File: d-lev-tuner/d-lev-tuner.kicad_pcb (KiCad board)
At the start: 4 copper layers, 88.7 x 68.4 mm, 40 parts, among them J1 S6B-PH-SM4-TB, U1 STP08CP05, U2 STP08CP05, U3 AP2112K-3.3, U4 STP08CP05, U5 DSM7TA56

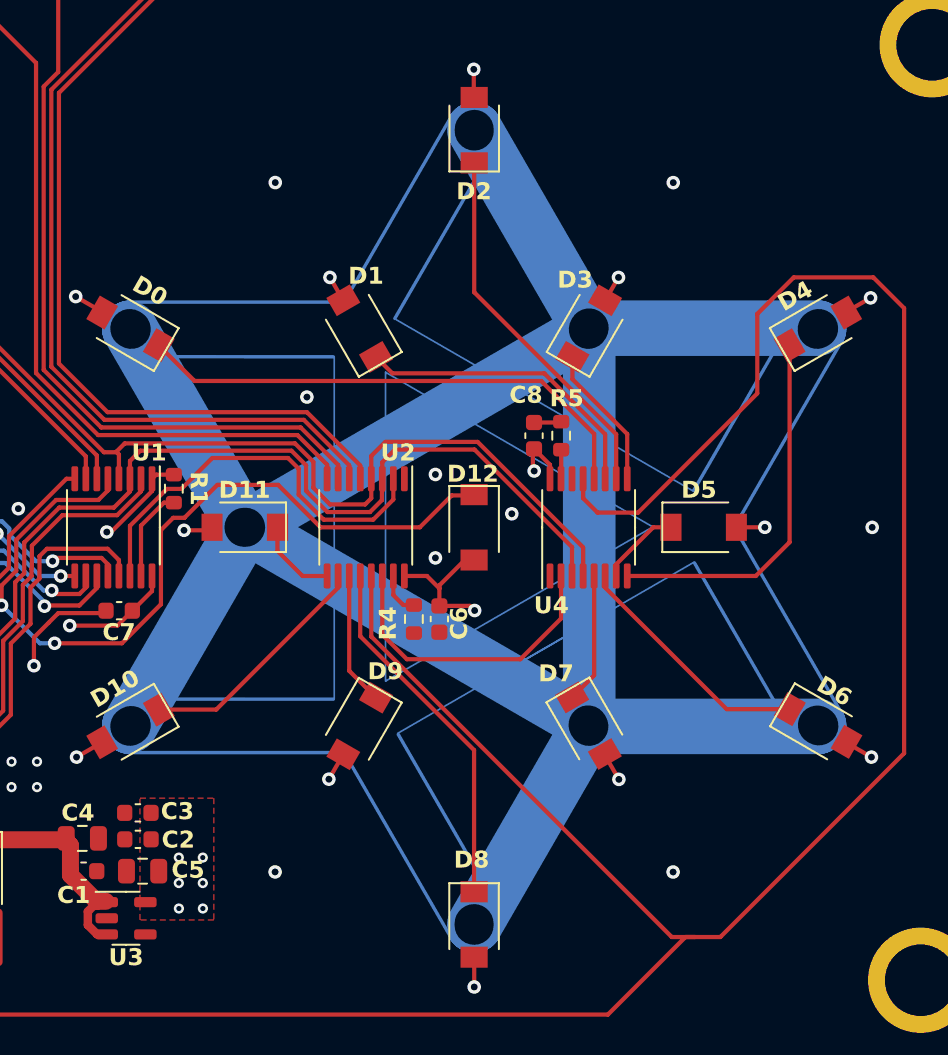
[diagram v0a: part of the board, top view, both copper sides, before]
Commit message: Add iBOMs and additional part numbers
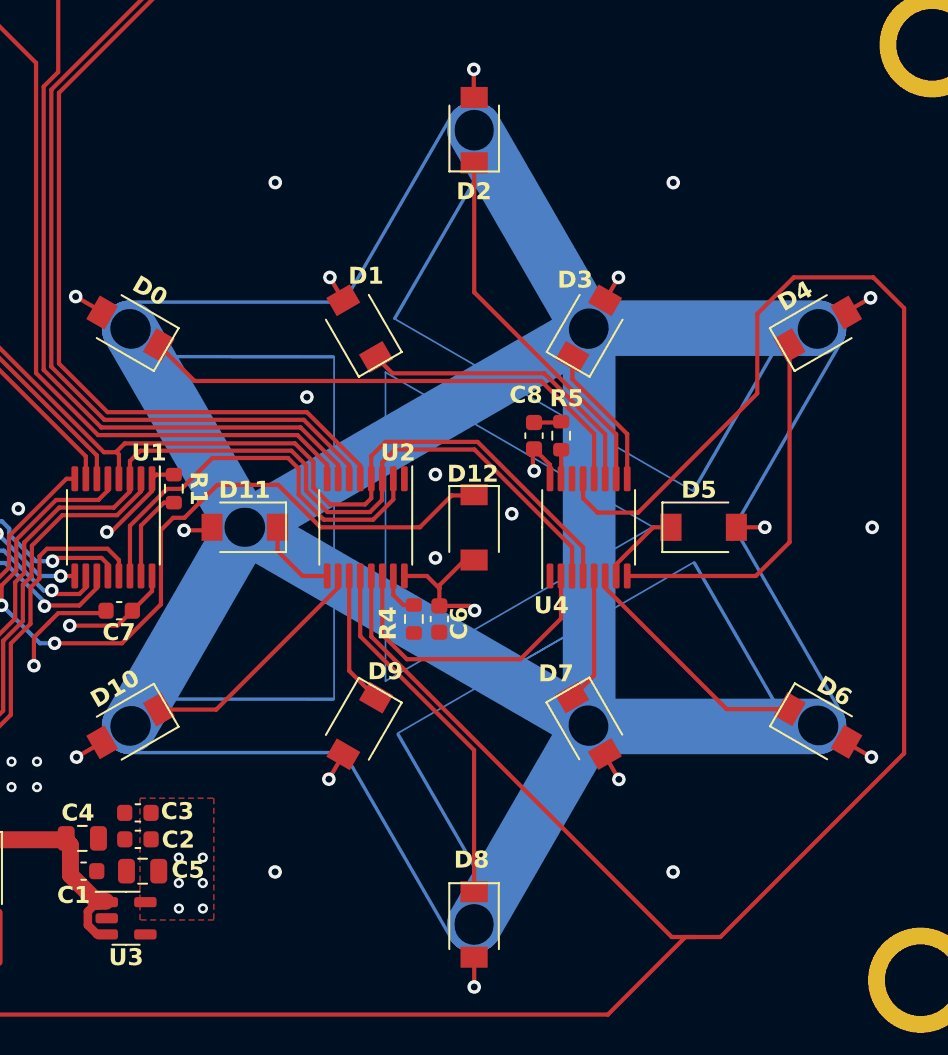
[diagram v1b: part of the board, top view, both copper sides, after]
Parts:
- C2, C6, C7, C8: value .1u -> 100n
